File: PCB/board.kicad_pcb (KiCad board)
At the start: 2 copper layers, 81.7 x 88.8 mm, 165 parts, among them J1 Micro_SD_Card, J10 Conn_01x10, J11 Conn_01x02, J12 Conn_02x04_Odd_Even, J13 Conn_01x02, J14 Conn_01x02, J15 Conn_01x03, J16 Conn_01x02, J17 Conn_01x05, J18 Conn_01x04, J19 Conn_01x04, J2 Conn_ARM_JTAG_SWD_10, J20 Conn_01x02, J21 Conn_01x03, J22 Conn_02x04_Odd_Even, J23 Conn_01x04, J24 Conn_01x04, J25 Conn_01x02, J26 Conn_01x03, J27 Conn_02x04_Odd_Even, J28 Conn_01x04, J29 Conn_01x04, J3 USB_C_Receptacle_USB2.0_14P, J30 Conn_01x02, J31 Conn_01x03, J32 Conn_01x02, J33 Conn_01x02, J34 Conn_01x02, J35 Conn_01x02, J36 Conn_01x02, J37 Conn_01x02, J4 Conn_01x04, J5 Conn_01x04, J6 Conn_01x02, J7 Conn_01x03, J8 Conn_02x04_Odd_Even, J9 Conn_01x10, Q1 IRLML6402, Q2 NMOS, Q3 NMOS, Q4 NMOS, Q5 Q_NMOS_GDS, Q7 Q_NMOS_GDS, SW1 SW_Push, SW2 SW_Push, U1 STM32H743VITx, U2 AP7361C, U4 TMC Stepstick, U5 TMC Stepstick, U6 TMC Stepstick, U7 TMC Stepstick, U8 AP63203WU, Y2 25 MHz

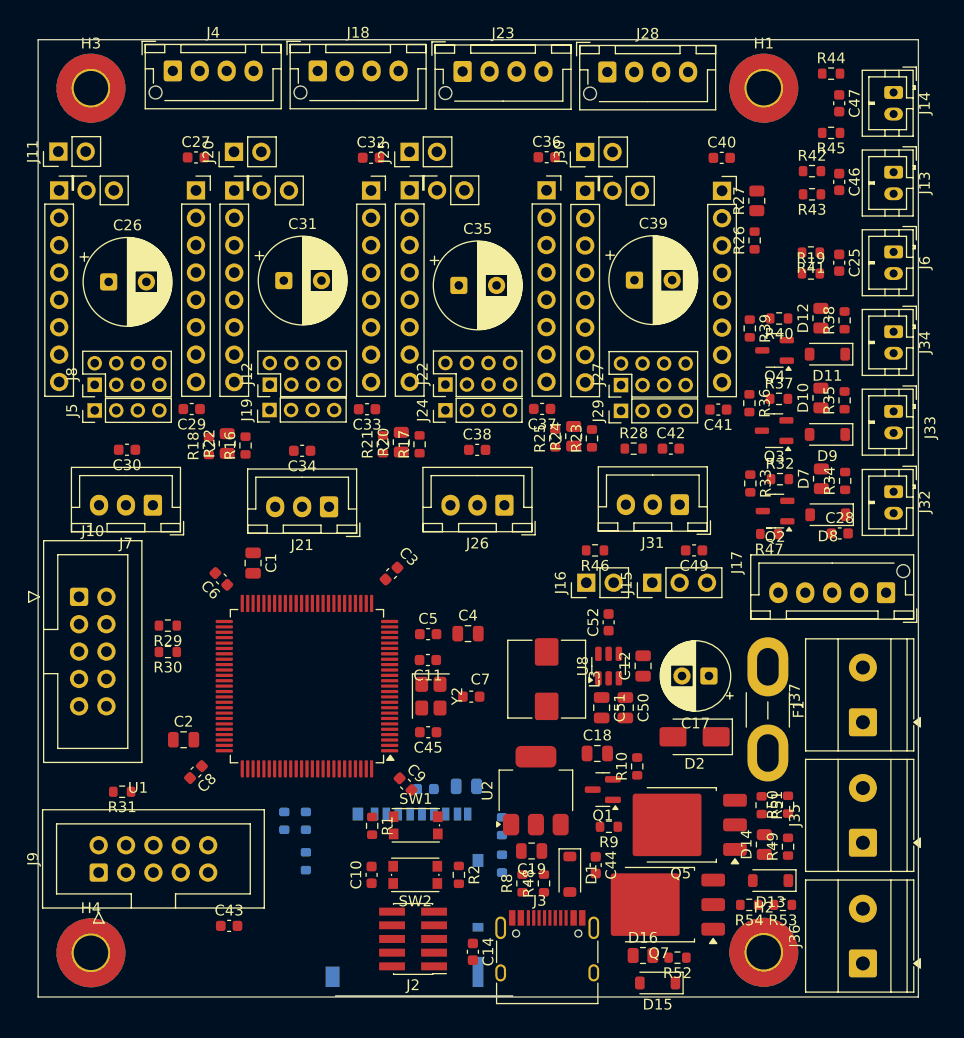
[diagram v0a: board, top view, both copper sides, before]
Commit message: fine tuning some stuff
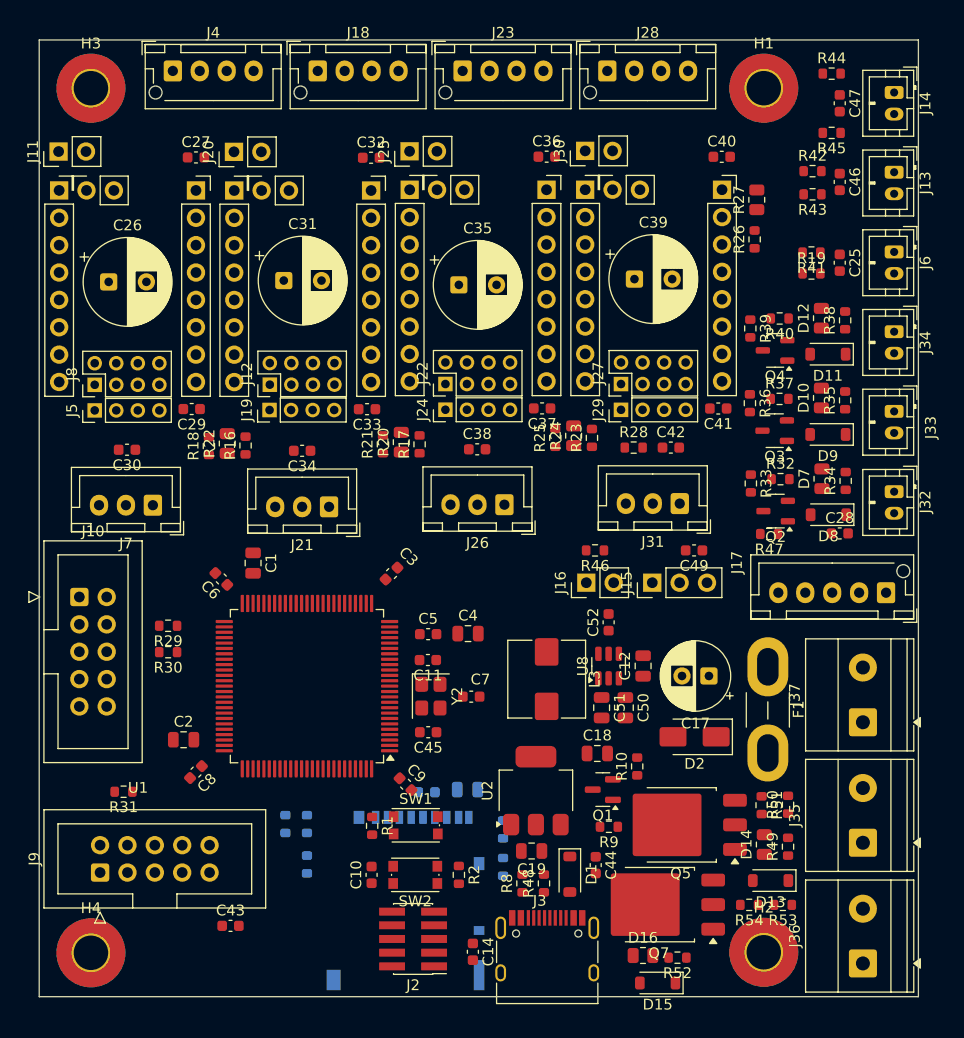
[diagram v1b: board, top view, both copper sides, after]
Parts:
- moved C15 0.32 mm to (189.6, 93.8)
- moved C16 0.32 mm to (193.4, 93.5)
- moved J1 0.32 mm to (187.7, 103.8)
- moved R3 0.32 mm to (176.5, 96.8)
- moved R4 0.32 mm to (178.5, 96.8)
- moved R5 0.32 mm to (178.5, 100.5)
- moved R6 0.32 mm to (196.7, 100.7)
- moved R7 0.32 mm to (196.7, 97.2)
- moved J9 0.13 mm to (159.3, 101.2)
- moved C43 0.13 mm to (171.4, 106.2)
- moved R31 0.13 mm to (161.5, 93.7)
- moved J31 0.10 mm to (213.1, 67.0)
- moved C41 0.10 mm to (216.7, 58.2)
- moved J27 0.10 mm to (207.7, 55.9)
- moved J30 0.10 mm to (204.3, 34.3)
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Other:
- board size 81.7 x 88.8 mm -> 81.6 x 88.8 mm
